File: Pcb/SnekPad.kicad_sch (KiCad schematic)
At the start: 15 parts, among them J1 OLED_128x32, SW1 RotaryEncoder_Switch, U1 Raspberry_Pi_Pico

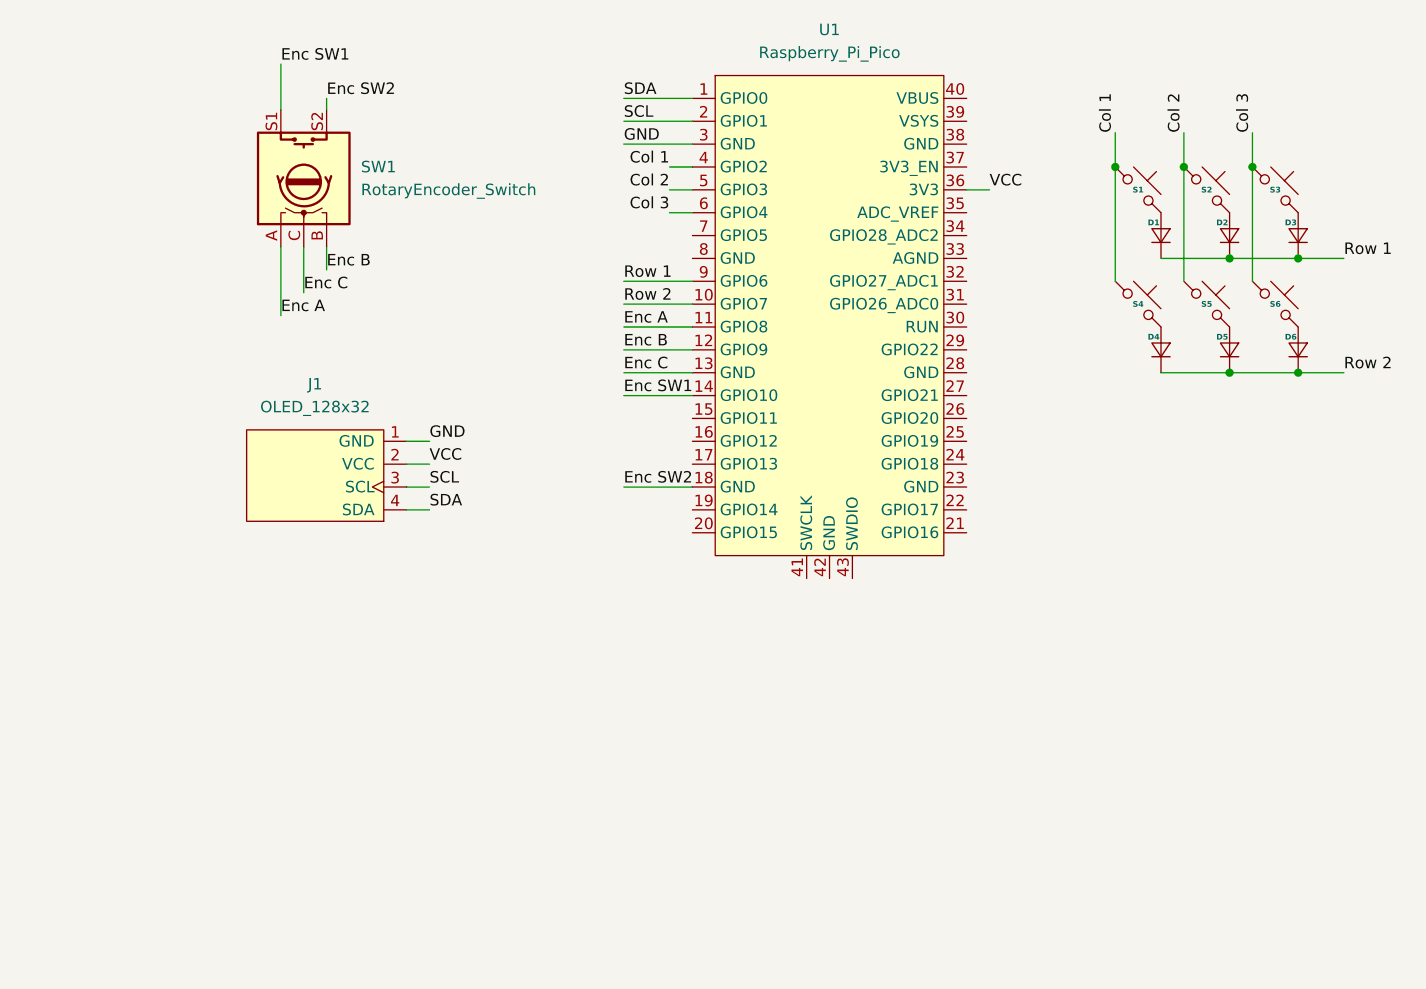
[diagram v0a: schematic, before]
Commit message: Update SnekPad.kicad_sch
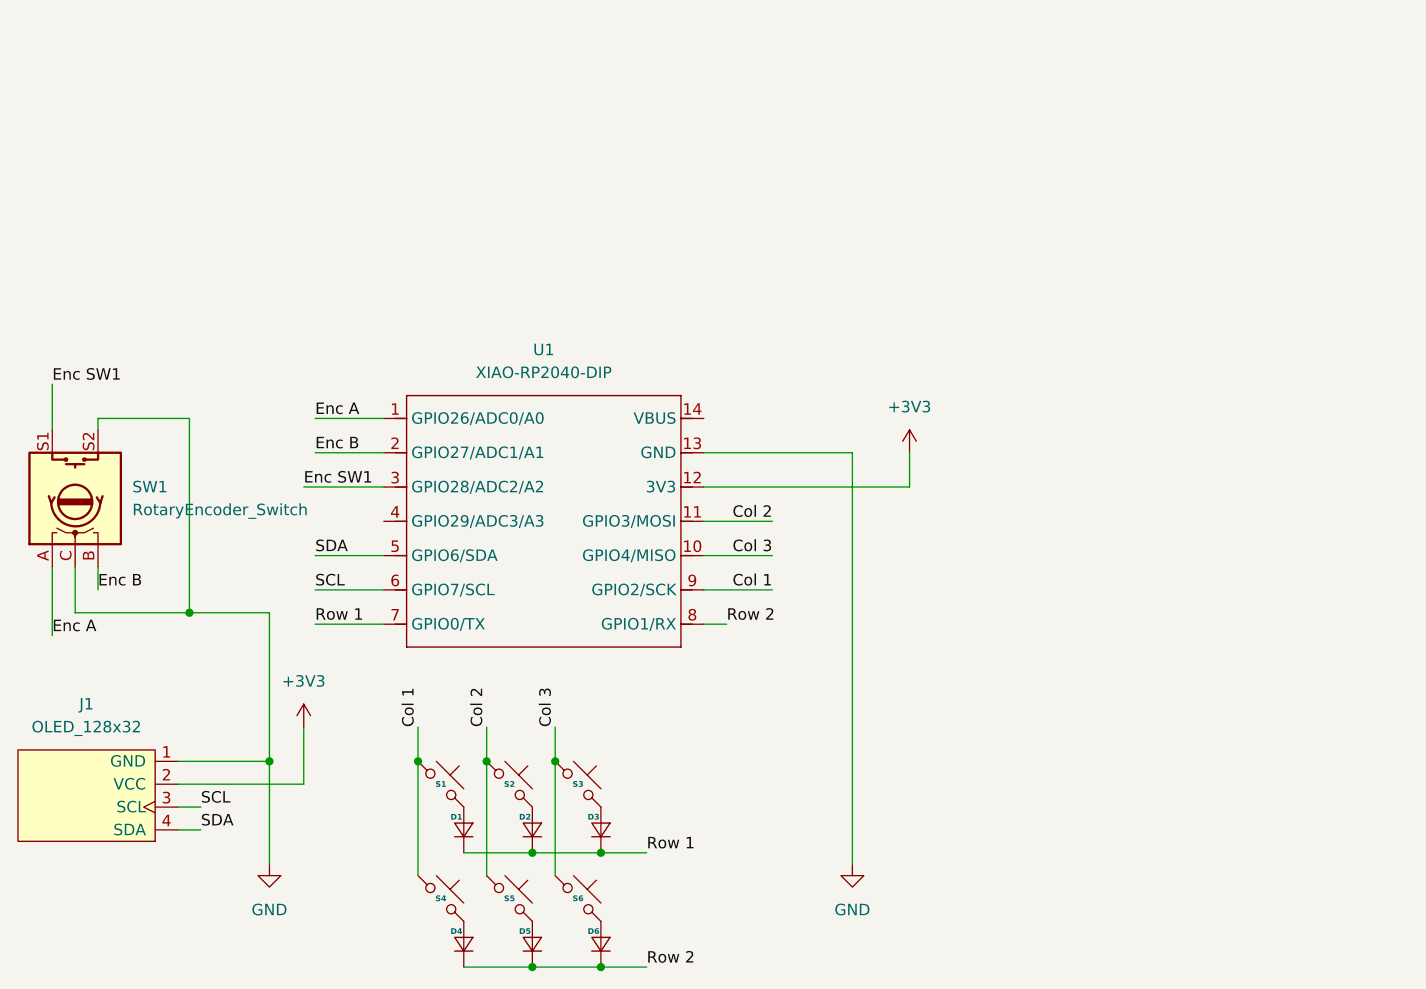
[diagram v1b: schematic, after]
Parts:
- removed U1: Raspberry_Pi_Pico, Module:RaspberryPi_Pico_Common_THT, symbol ScottoKeebs:MCU_Raspberry_Pi_Pico
- added U1: XIAO-RP2040-DIP, OPL Library:XIAO-RP2040-DIP, symbol OPL Library:XIAO-RP2040-DIP
- J1: footprint ScottoKeebs_Components:OLED_128x32 -> Hackclub Footprints:OLED_0.91_128x32
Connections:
- net Enc C is gone; now on net GND: SW1.C
- net Enc SW2 is gone; now on net GND: SW1.S2
- net Col 1: now also U1.9 (GPIO2/SCK)
- net Col 2: now also U1.11 (GPIO3/MOSI)
- net Col 3: now also U1.10 (GPIO4/MISO)
- net Enc A: now also U1.1 (GPIO26/ADC0/A0)
- net Enc B: now also U1.2 (GPIO27/ADC1/A1)
- net Enc SW1: now also U1.3 (GPIO28/ADC2/A2)
- net GND: now also U1.13 (GND)
- net Row 1: now also U1.7 (GPIO0/TX)
- net Row 2: now also U1.8 (GPIO1/RX)
- net SCL: now also U1.6 (GPIO7/SCL)
- net SDA: now also U1.5 (GPIO6/SDA)
- net VCC renamed +3V3
- net +3V3: now also U1.12 (3V3)
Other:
- moved on the sheet: D1, D2, D3, D4, D5, D6, S1, S2, S3, S4, S5, S6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
